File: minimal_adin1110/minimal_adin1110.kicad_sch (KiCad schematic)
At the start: 73 parts, among them J1 CLP-114-02-G-D-BE, J2 CLP-102-02-G-D-BE, J3 CLP-102-02-G-D-BE, J4 CLP-102-02-G-D-BE, J5 CLP-103-02-G-D-BE, U1 ADIN1110CCPZ, Y1 25.0000MHz

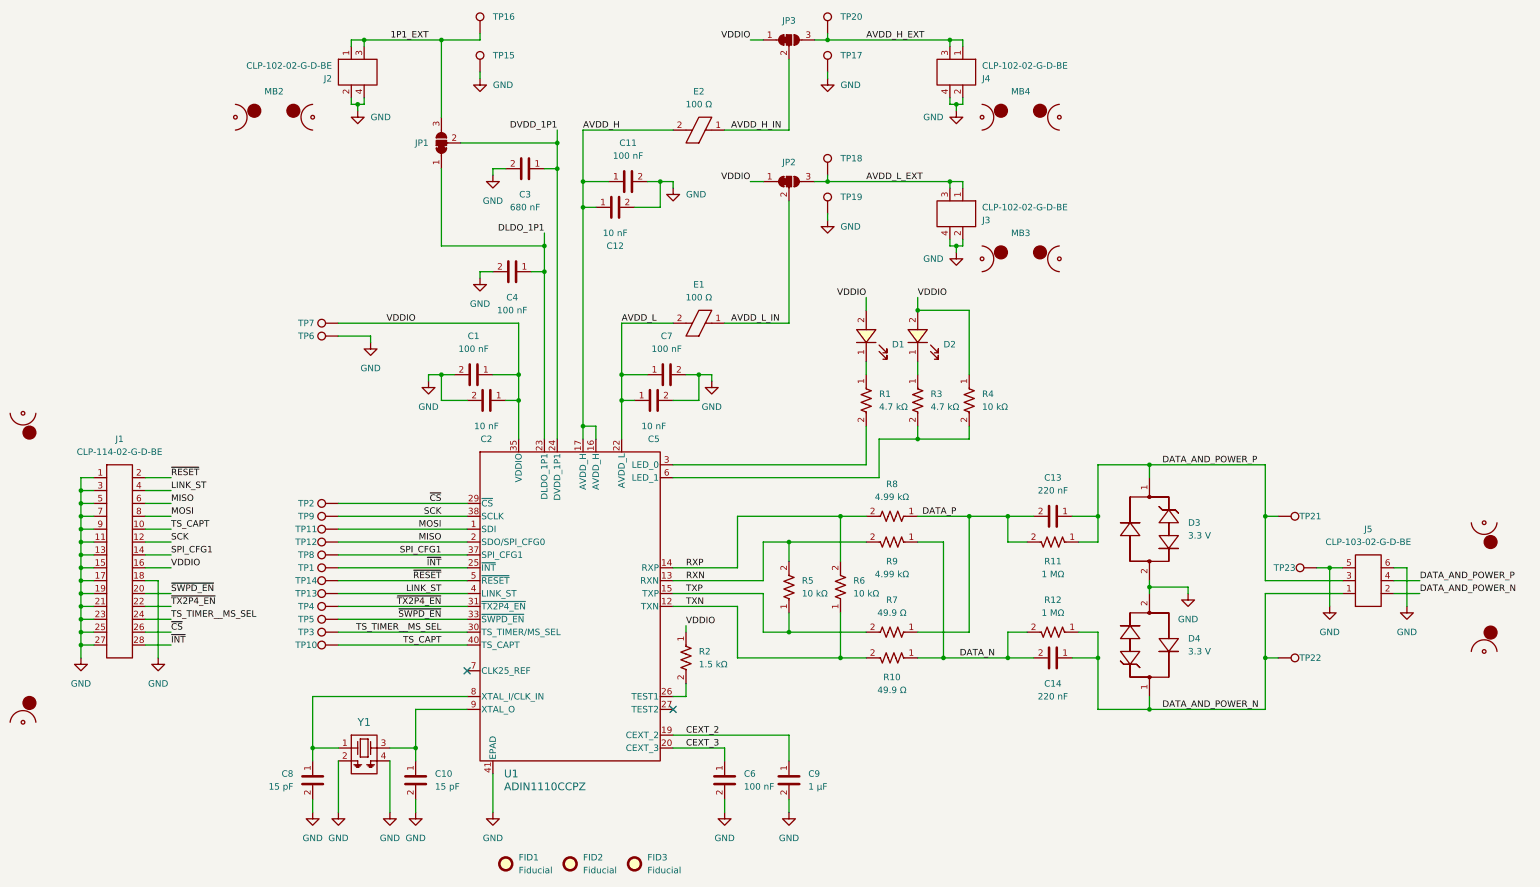
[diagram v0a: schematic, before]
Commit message: Switch to KiCad 9
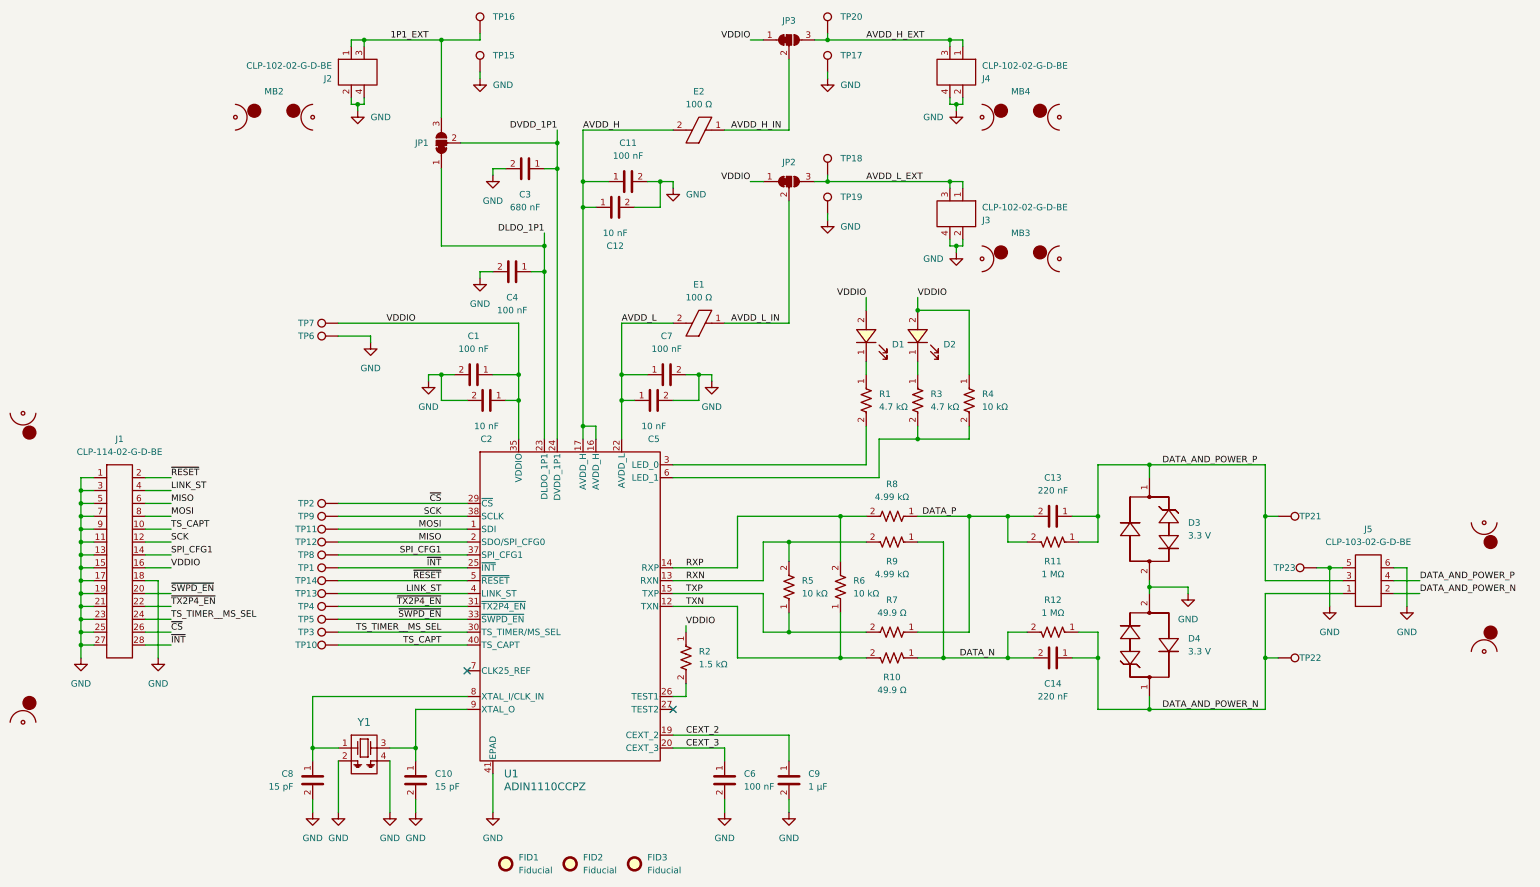
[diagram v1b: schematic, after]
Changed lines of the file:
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@@
 (kicad_sch
-	(version 20231120)
+	(version 20250114)
 	(generator "eeschema")
-	(generator_version "8.0")
+	(generator_version "9.0")
 	(paper "A3")
 	(junction
@@
 		)
 	)
+	(embedded_fonts no)
 )
